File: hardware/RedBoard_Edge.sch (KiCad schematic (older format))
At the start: 72 parts, among them J1 CONN_025MM, J17 QWIIC_CONNECTORJS-1MM, J18 QWIIC_CONNECTORJS-1MM, J2 CONN_03X2SMT, J20 POWER_JACKSMD, J3 CONN_02, J4 USB_MICRO-B_FEMALE-SMT, J5 CONN_04, J6 CONN_04, J7 CONN_02, J8 CONN_02, Q1 MOSFET_PCH-SI2309DS, Q2 MOSFET-NCH-BSS138, Q3 MOSFET-NCH-BSS138, U1 CH340GSMD, U2 V_REG_MIC52053.3V, U3 Standoff_Grounding, U4 ATMEGA328P_TQFP, U5 Standoff_Grounding, U6 V_REG_LM1117SOT223, Y1 RESONATOR-16MHZSMD_3.2X1.3, Y2 CRYSTAL-12MHZ\"

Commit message: Post Design review changes
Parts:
- removed 5V1, ADC1, GND1: CONN_06SILK_FEMALE_PTH, symbol CONN_06SILK_FEMALE_PTH
- removed J18: QWIIC_CONNECTORJS-1MM, symbol QWIIC_CONNECTORJS-1MM
- removed J3, J7, J8: CONN_02, symbol CONN_02
- added 5V1, 5V4, ADC1, ADC4, GND1, GND4: CONN_04, Connectors:1X04_NO_SILK, symbol CONN_04
- 5V2, 5V3, GND2, GND3: footprint (none) -> Connectors:1X04_NO_SILK
- C1, C10, C11, C12, C2, C4, C7, C8, C9: footprint Capacitors:0603 -> (none)
- C3, C6: footprint Capacitors:EIA3216 -> (none)
- C5: footprint Capacitors:EIA3528 -> (none)
- D1: footprint Silicon-Standard:SMA-DIODE -> (none)
- D2, D3, D4, D5: footprint LED:LED_550_T1-.75_RT_ANG_PCB -> (none)
- F1: footprint Fuses:1206 -> (none)
- FD1, FD2, FD3, FD4: footprint Aesthetics:FIDUCIAL-MICRO -> (none)
- H1, H2: footprint Hardware:STAND-OFF-TIGHT -> (none)
- J20: footprint (none) -> Connectors:POWER_JACK_SMD_GND
- JP1, JP2: footprint Jumpers:SMT-JUMPER_2_NO_NO-SILK -> (none)
- Q1, Q2, Q3: footprint Silicon-Standard:SOT23-3 -> (none)
- R1, R10, R14, R15, R2, R3, R4, R5, R6, R7, R8, R9: footprint Resistors:0603 -> (none)
- S1: footprint Switches:TACTILE_SWITCH_PTH_RIGHT_ANGLE_KIT -> (none)
- S2: footprint Switches:TACTILE_SWITCH_SMD_RIGHT_ANGLE -> (none)
- U1: footprint Silicon-Standard:SO16 -> (none)
- U2: footprint Silicon-Standard:SOT23-5 -> (none)
- U3, U5: footprint Hardware:STANDOFF_GROUNDING -> (none)
- U4: footprint Silicon-Standard:TQFP32-08 -> (none)
- U6: footprint Silicon-Standard:SOT223 -> (none)
- Y1: footprint Clocks:RESONATOR-SMD-3.2X1.3 -> (none)
- Y2: footprint Clocks:CRYSTAL-SMD-5X3.2-4PAD -> (none)
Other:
- moved on the sheet: S2

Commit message: forgot to save before commit
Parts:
- added LOGO1: SFE_LOGO_NAME_FLAME.1_INCH, SFE_LOGO_NAME_FLAME_.1, symbol SFE_LOGO_NAME_FLAME.1_INCH
- added LOGO2: OSHW-LOGOS, OSHW-LOGO-S, symbol OSHW-LOGOS
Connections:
- wire segments 246 -> 247
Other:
- note added: "Design by: Nick Poole"
- note added: "Revised by: Andy England"
- note added: "v01"

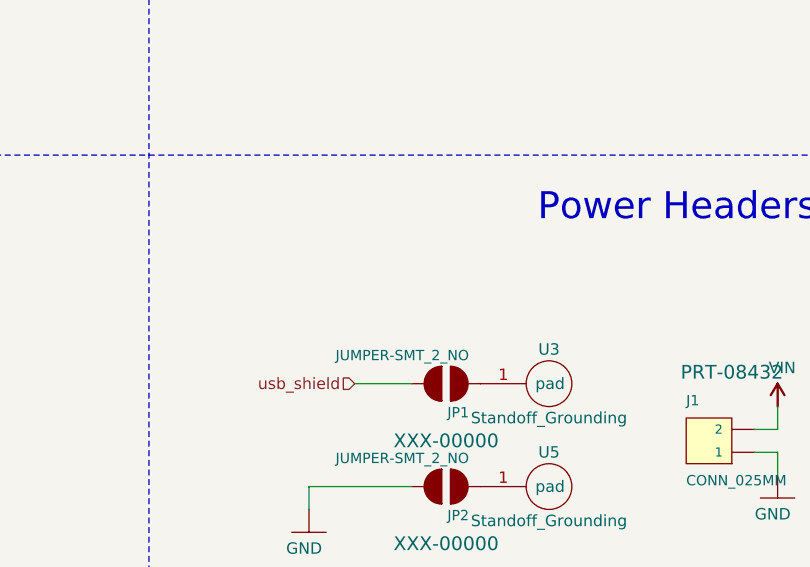
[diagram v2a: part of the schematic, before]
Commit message: QC Double Check Issues
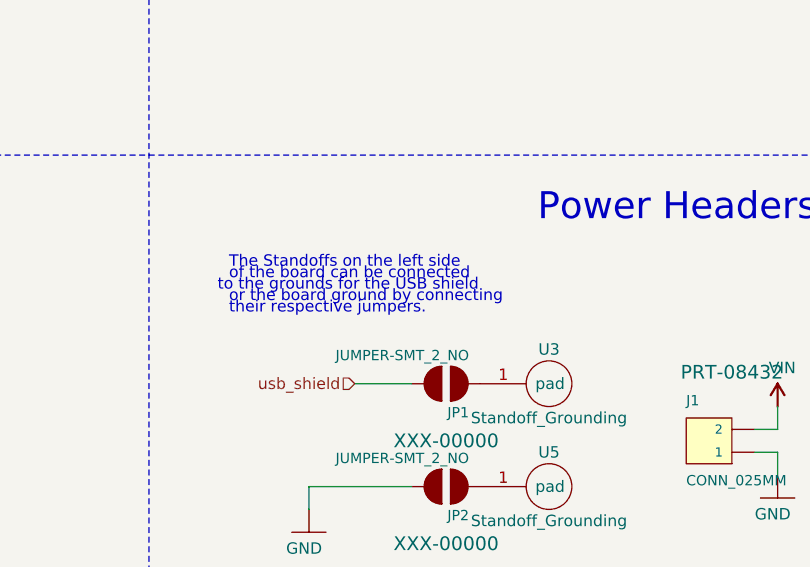
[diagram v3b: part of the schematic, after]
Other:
- note added: "The Standoffs on the left side"
- note added: "of the board can be connected"
- note added: "or the board ground by connecting"
- note added: "their respective jumpers."
- note added: "to the grounds for the USB shield"
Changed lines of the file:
@@
 Text Notes 15950 10350 0    50   ~ 0
 v01
+Text Notes 6200 6050 0    50   ~ 0
+The Standoffs on the left side
+Text Notes 6200 6100 0    50   ~ 0
+of the board can be connected
+Text Notes 6150 6150 0    50   ~ 0
+ to the grounds for the USB shield
+Text Notes 6200 6200 0    50   ~ 0
+or the board ground by connecting
+Text Notes 6200 6250 0    50   ~ 0
+their respective jumpers.
 $EndSCHEMATC
